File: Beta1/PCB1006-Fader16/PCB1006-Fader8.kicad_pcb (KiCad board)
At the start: 2 copper layers, 199 x 30.9 mm, 43 parts, among them U1000 MCP3008T-I/SL, U2 MCP3008T-I/SL

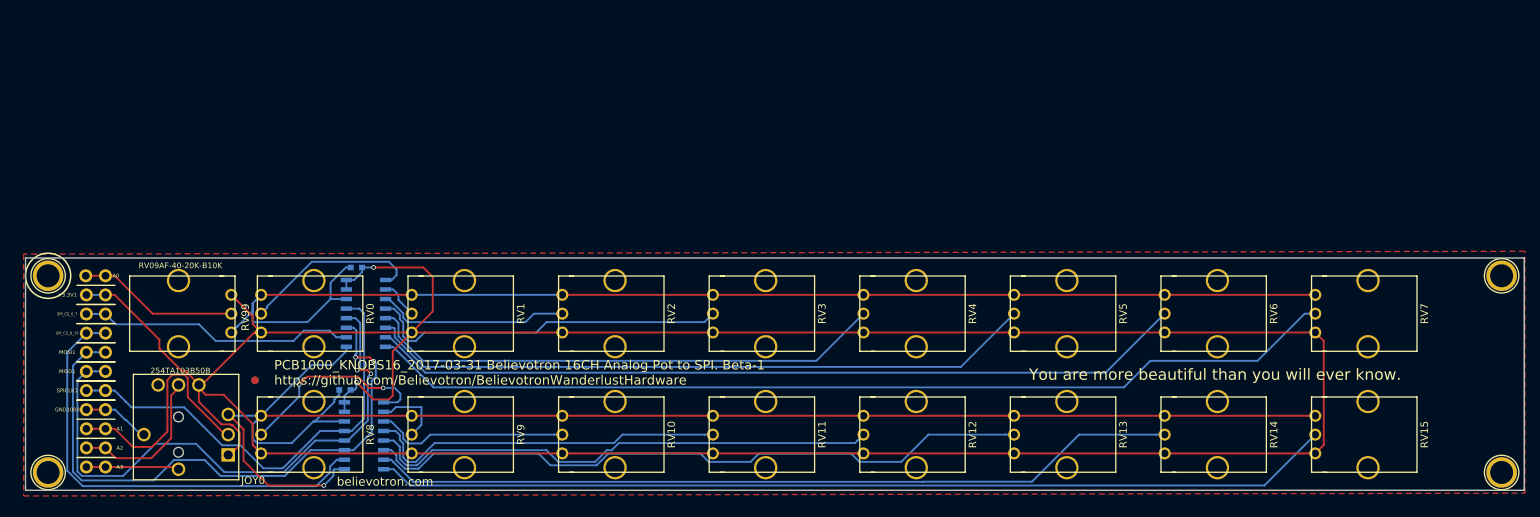
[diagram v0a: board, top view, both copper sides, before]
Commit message: Routing complete
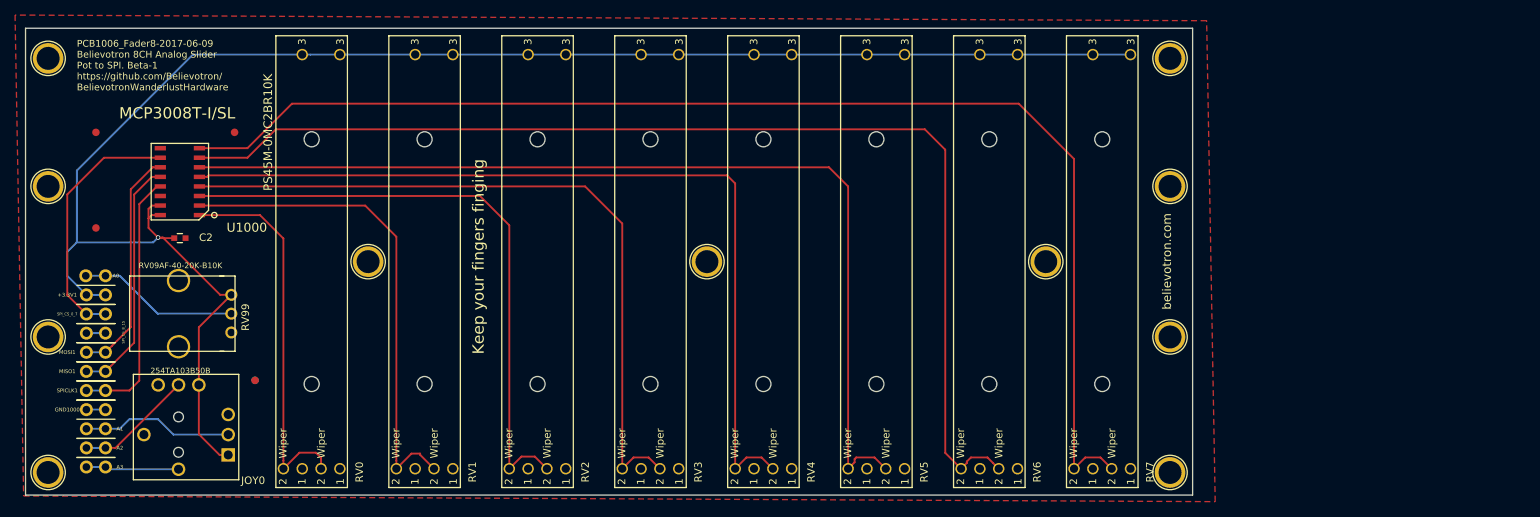
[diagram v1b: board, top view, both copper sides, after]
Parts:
- removed C1000: 0.1u, Capacitors_SMD:C_0603
- removed RV10, RV11, RV12, RV13, RV14, RV15, RV8, RV9: POT, Liberry:RV09AF-40-20K-B10K
- removed U2: MCP3008T-I/SL, Liberry:SOIC-16
- added REF**: Fiducial_1mm_Dia_2.54mm_Outer_CopperTop, Fiducials:Fiducial_1mm_Dia_2.54mm_Outer_CopperTop, F.Cu at (9.35, -35.5)
- added REF**: Fiducial_1mm_Dia_2.54mm_Outer_CopperTop, Fiducials:Fiducial_1mm_Dia_2.54mm_Outer_CopperTop, F.Cu at (9.35, -48.2)
- added REF**: Fiducial_1mm_Dia_2.54mm_Outer_CopperTop, Fiducials:Fiducial_1mm_Dia_2.54mm_Outer_CopperTop, F.Cu at (27.8, -48.2)
- added REF**: 1pin, Connect:1pin, F.Cu at (152.0, -21.0)
- added REF**: 1pin, Connect:1pin, F.Cu at (135.5, -31.0)
- added REF**: 1pin, Connect:1pin, F.Cu at (45.5, -31.0)
- added REF**: 1pin, Connect:1pin, F.Cu at (90.5, -31.0)
- added REF**: 1pin, Connect:1pin, F.Cu at (152.0, -41.0)
- added REF**: 1pin, Connect:1pin, F.Cu at (3.00, -21.0)
- added REF**: 1pin, Connect:1pin, F.Cu at (3.00, -41.0)
- C2, U1000: moved to F.Cu
- RV0, RV1, RV2, RV3, RV4, RV5, RV6, RV7: footprint Liberry:RV09AF-40-20K-B10K -> Liberry:LINEAR_POT_TT_ELECTRONICS_PS45M
- moved REF** 52.7 mm to (152.0, -58.0)
- moved REF** 44.0 mm to (152.0, -3.00)
- moved RV7 36.0 mm to (143.0, -31.0), turned to 90 degrees
- moved RV6 31.1 mm to (128.0, -31.0), turned to 90 degrees
- moved U1000 30.3 mm to (20.5, -41.6), turned to 90 degrees
- moved C2 29.8 mm to (20.5, -34.1), turned to 0 degrees
- moved REF** 28.9 mm to (3.00, -58.0)
- moved RV5 26.2 mm to (113.0, -31.0), turned to 90 degrees
- moved RV4 21.4 mm to (98.0, -31.0), turned to 90 degrees
- moved RV3 16.8 mm to (83.0, -31.0), turned to 90 degrees
- moved RV2 12.4 mm to (68.0, -31.0), turned to 90 degrees
- moved RV1 8.71 mm to (53.0, -31.0), turned to 90 degrees
- moved RV0 6.91 mm to (38.0, -31.0), turned to 90 degrees
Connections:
- RV0 pad 1: +3V3 -> GND
- RV0 pad 3: GND -> +3V3
- RV1 pad 1: +3V3 -> GND
- RV1 pad 3: GND -> +3V3
- RV2 pad 1: +3V3 -> GND
- RV2 pad 3: GND -> +3V3
- RV3 pad 1: +3V3 -> GND
- RV3 pad 3: GND -> +3V3
- RV4 pad 1: +3V3 -> GND
- RV4 pad 3: GND -> +3V3
- RV5 pad 1: +3V3 -> GND
- RV5 pad 3: GND -> +3V3
- RV6 pad 1: +3V3 -> GND
- RV6 pad 3: GND -> +3V3
- RV7 pad 1: +3V3 -> GND
- RV7 pad 3: GND -> +3V3
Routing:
- net GND: track 384.2 -> 2.54 mm, vias 1 -> 0
- net +3V3: track 406.8 -> 226.2 mm, vias 2 -> 1
- net /P15: track 127.4 -> 0.00 mm
- net /P14: track 107.6 -> 0.00 mm
- net /P13: track 90.1 -> 0.00 mm
- net /P12: track 69.0 -> 0.00 mm
- net /P1: track 5.24 -> 65.4 mm
- net /CS_LED_8_15: track 61.4 -> 2.54 mm
- net /P2: track 25.6 -> 81.4 mm
- net /MOSI: track 81.3 -> 30.7 mm, vias 2 -> 0
- net /P3: track 48.2 -> 97.0 mm
- net /P11: track 48.4 -> 0.00 mm
- net /P4: track 69.5 -> 115.8 mm
- net /MISO: track 78.3 -> 32.1 mm, vias 2 -> 0
- net /P6: track 108.7 -> 151.3 mm
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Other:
- board size 199 x 30.9 mm -> 155 x 62 mm
- board text added: "Keep your fingers finging"
- board text added: "PCB1006_Fader8-2017-06-09 Believotron 8CH Analog Slider Pot to SPI. Beta-1 https://github.com/Believotron/ BelievotronWanderlustHardware"
- board text added: "PS45M-0MC2BR10K"
- board text removed: "PCB1000_KNOBS16_2017-03-31 Believotron 16CH Analog Pot to SPI. Beta-1 https://github.com/Believotron/BelievotronWanderlustHardware"
- board text removed: "You are more beautiful than you will ever know."
